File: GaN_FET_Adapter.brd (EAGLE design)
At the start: 22.9 x 20.3 mm, 15 parts

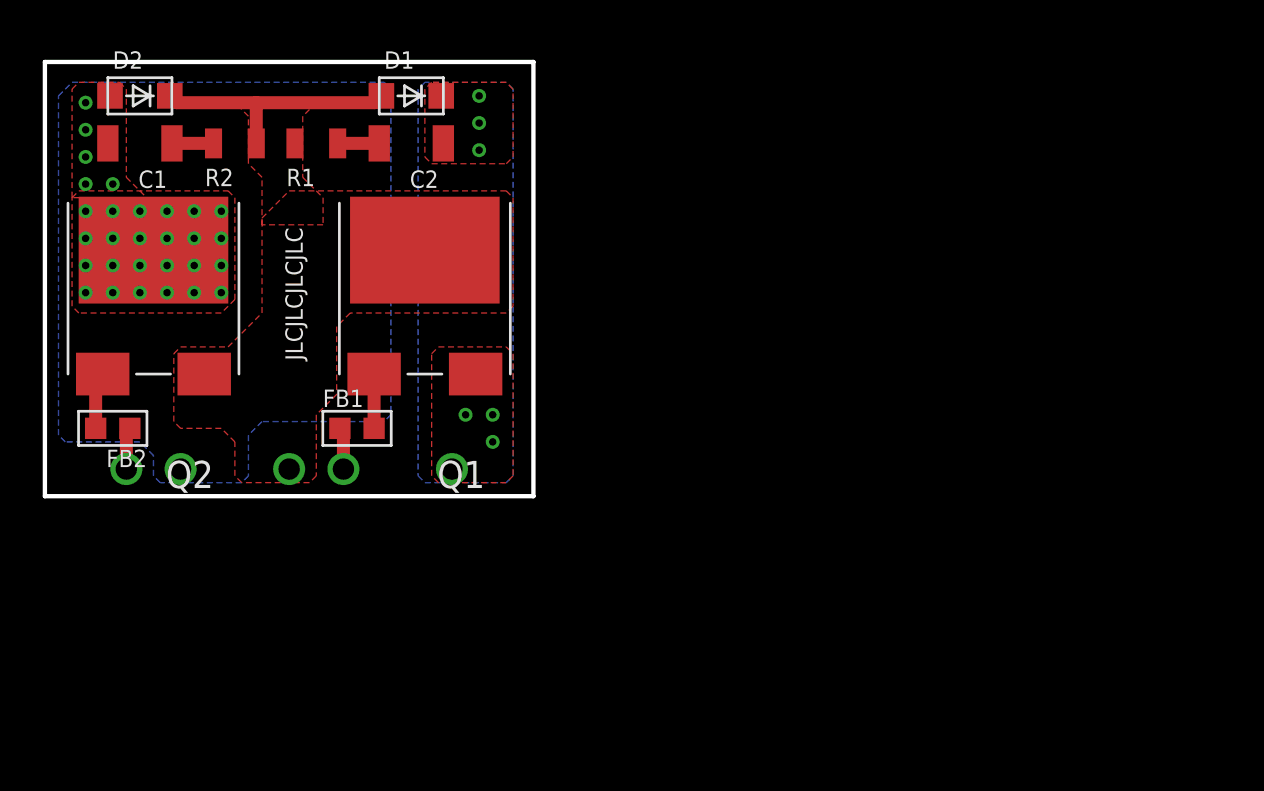
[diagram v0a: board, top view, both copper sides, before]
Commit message: 発注
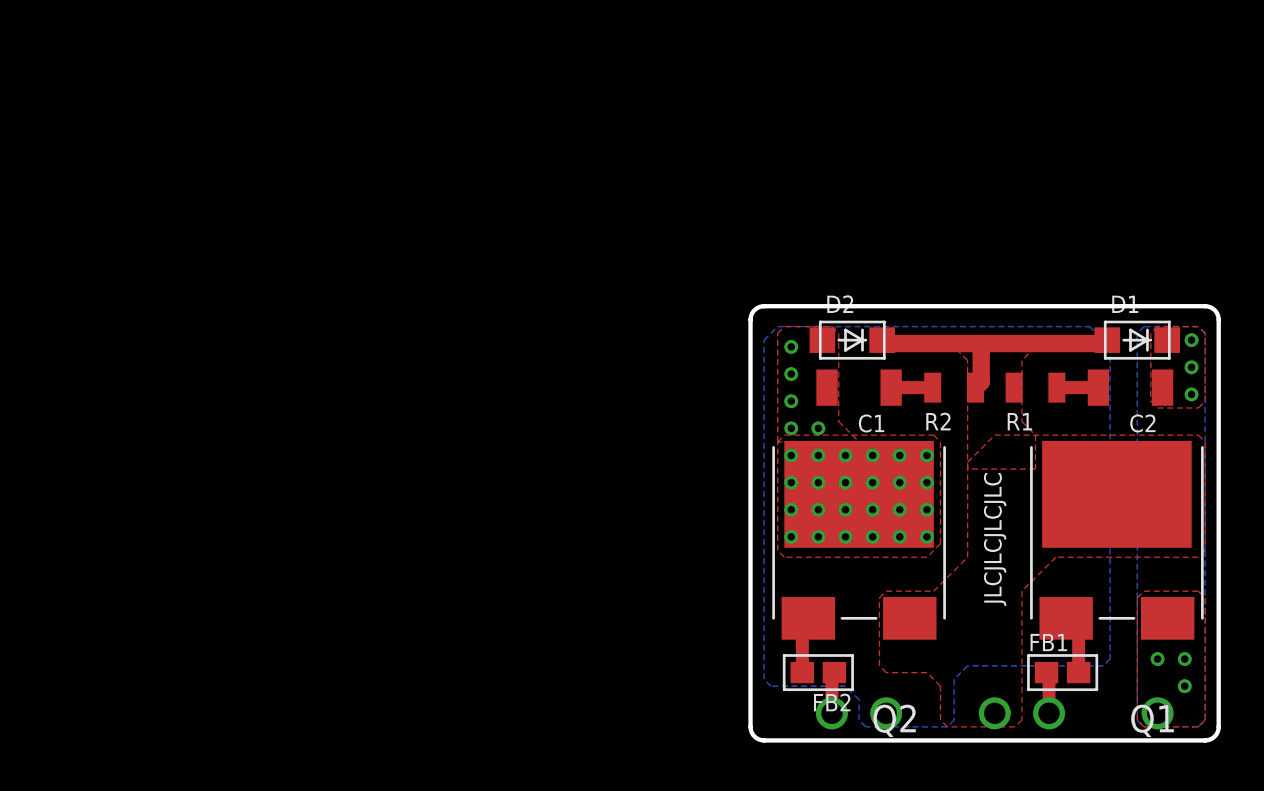
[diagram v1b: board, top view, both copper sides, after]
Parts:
- moved D1 35.8 mm to (18.1, 18.7)
- moved C1 35.5 mm to (5.08, 16.5)
- moved C2 35.5 mm to (17.8, 16.5)
- moved R1 35.5 mm to (13.3, 16.5)
- moved R2 35.5 mm to (9.53, 16.5)
- moved D2 35.2 mm to (4.76, 18.7)
- moved Q2 34.9 mm to (5.08, 5.71)
- moved TP1 34.9 mm to (19.1, 1.27)
- moved TP3 34.9 mm to (6.35, 1.27)
- moved TP4 34.9 mm to (3.81, 1.27)
- moved TP5 34.9 mm to (14.0, 1.27)
- moved FB1 34.9 mm to (14.6, 3.17)
- moved FB2 34.9 mm to (3.17, 3.17)
- moved TP2 34.9 mm to (11.4, 1.27)
- moved Q1 34.3 mm to (17.1, 5.71)
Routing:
- net SW: track 12.1 -> 12.8 mm
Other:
- board size 22.9 x 20.3 mm -> 21.9 x 20.3 mm
